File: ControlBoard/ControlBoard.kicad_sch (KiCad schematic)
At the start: 30 parts

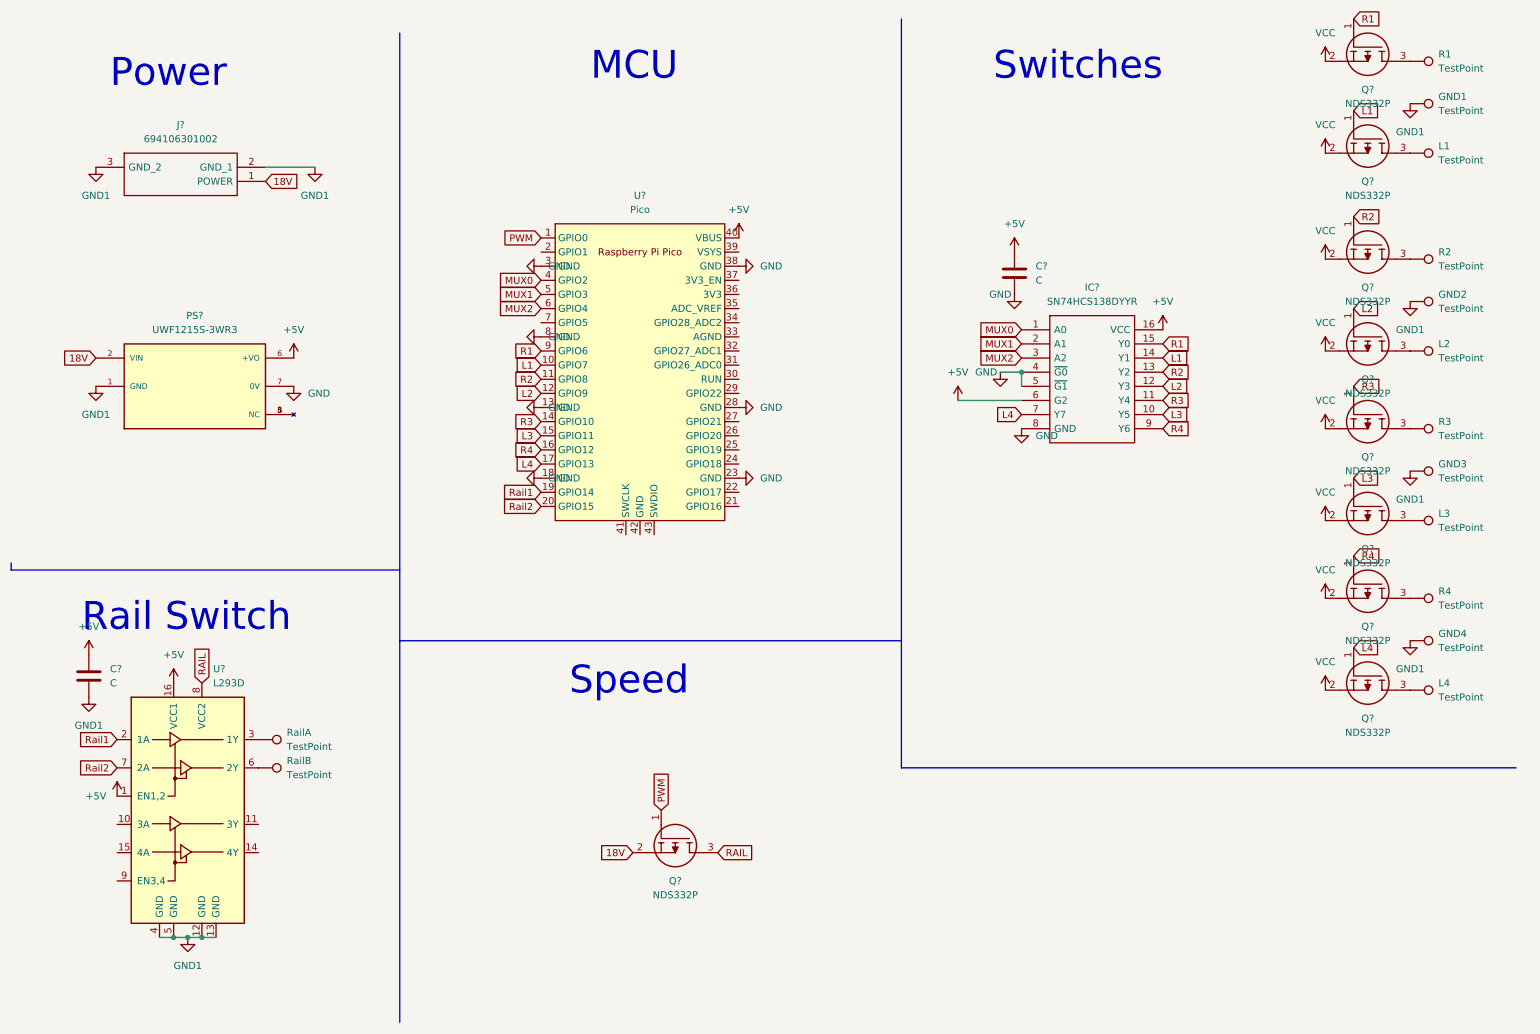
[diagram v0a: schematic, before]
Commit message: Finalized layout
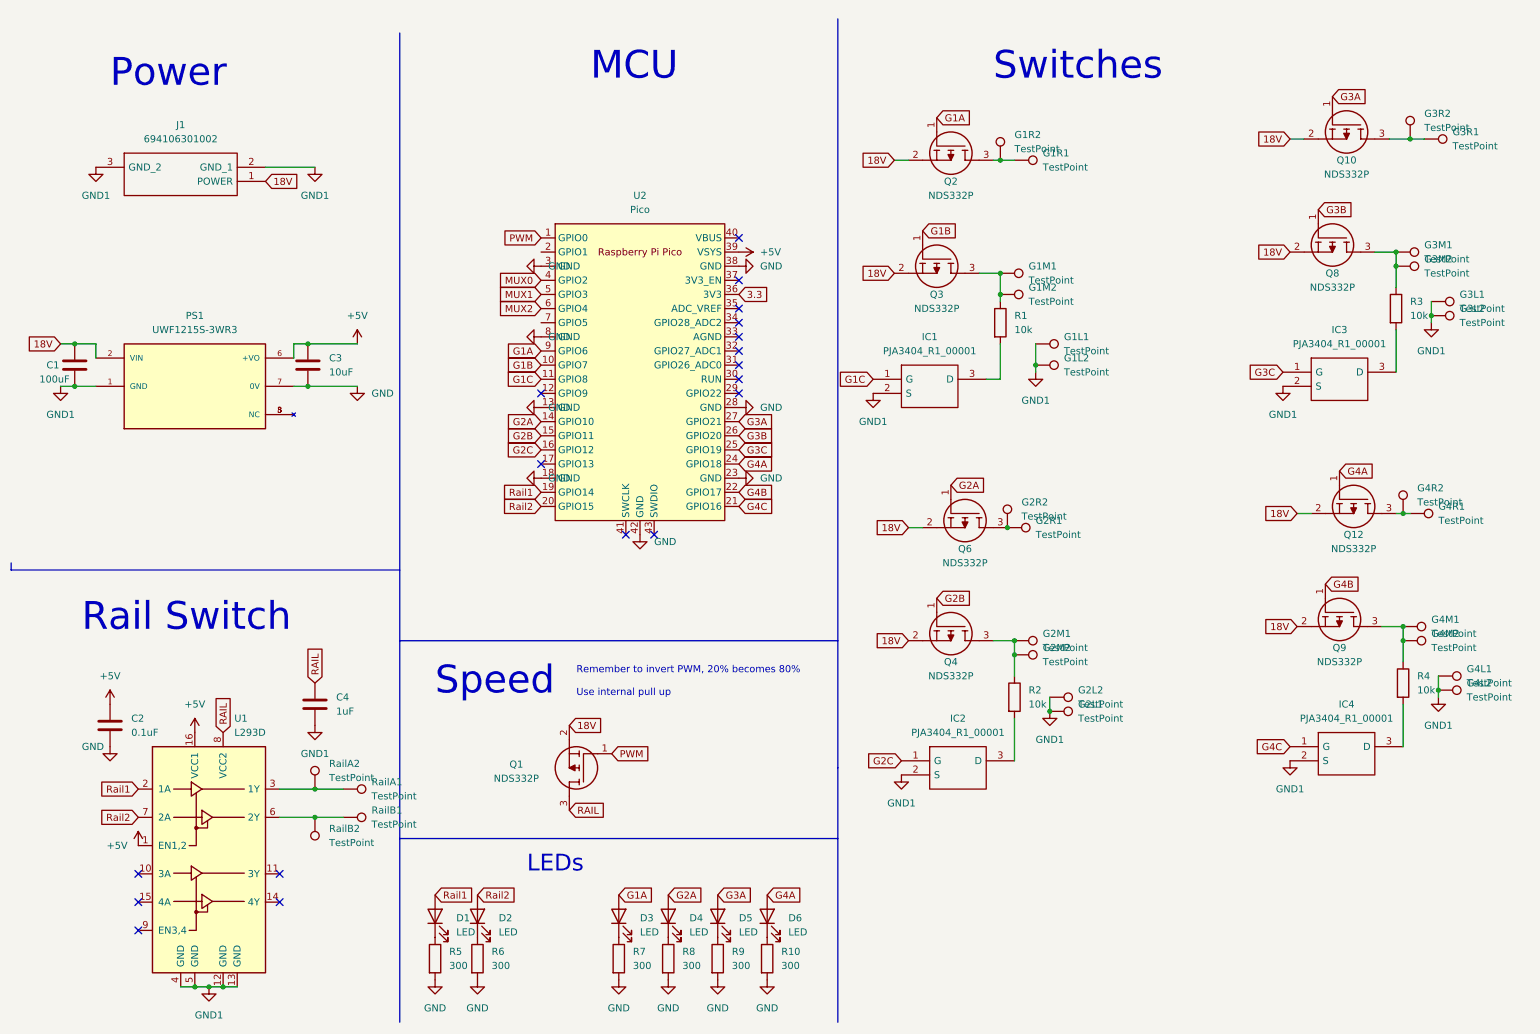
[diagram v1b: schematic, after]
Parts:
- removed C?: C, symbol Device:C
- removed GND2, GND3, GND4, L2, L3, L4, R2, R3, R4: TestPoint, symbol Connector:TestPoint
- removed IC?: SN74HCS138DYYR, SOP50P326X110-16N, symbol SamacSys_Parts:SN74HCS138DYYR
- removed Q? (x7): NDS332P, SOT95P237X112-3N, symbol SamacSys_Parts:NDS332P
- added C1: 100uF, Capacitor_THT:CP_Radial_D10.0mm_P7.50mm, symbol Device:C
- added C3: 10uF, Capacitor_THT:CP_Radial_D10.0mm_P7.50mm, symbol Device:C
- added C4: 1uF, Capacitor_THT:CP_Radial_D10.0mm_P7.50mm, symbol Device:C
- added D1, D2, D3, D4, D5, D6: LED, LED_THT:LED_D3.0mm, symbol Device:LED
- added G1L2, G1M2, G1R2, G2L1, G2L2, G2M1, G2M2, G2R1, G2R2, G3L1, G3L2, G3M1, G3M2, G3R1, G3R2, G4L1, G4L2, G4M1, G4M2, G4R1, G4R2, RailA2, RailB2: TestPoint, TestPoint:TestPoint_Pad_2.5x2.5mm, symbol Connector:TestPoint
- added IC1, IC2, IC3, IC4: PJA3404_R1_00001, SamacSys_Parts:SOT95P240X110-3N, symbol SamacSys_Parts:PJA3404_R1_00001
- added Q10, Q12, Q3, Q4, Q6, Q8, Q9: NDS332P, SamacSys_Parts:SOT95P237X112-3N, symbol SamacSys_Parts:NDS332P
- added R1, R2, R3, R4: 10k, Resistor_THT:R_Axial_DIN0204_L3.6mm_D1.6mm_P7.62mm_Horizontal, symbol Device:R
- added R10, R5, R6, R7, R8, R9: 300, Resistor_THT:R_Axial_DIN0204_L3.6mm_D1.6mm_P7.62mm_Horizontal, symbol Device:R
- C2: renamed from C?; value C -> 0.1uF; footprint (none) -> Capacitor_THT:CP_Radial_D10.0mm_P7.50mm
- G1L1: renamed from L1; footprint (none) -> TestPoint:TestPoint_Pad_2.5x2.5mm
- G1M1: renamed from GND1; footprint (none) -> TestPoint:TestPoint_Pad_2.5x2.5mm
- G1R1: renamed from R1; footprint (none) -> TestPoint:TestPoint_Pad_2.5x2.5mm
- J1: renamed from J?; footprint 694106301002_1 -> SamacSys_Parts:694106301002_1
- PS1: renamed from PS?; footprint CONV_UWF1215S-3WR3 -> UWF1215S-3WR3:CONV_UWF1215S-3WR3
- Q1, Q2: renamed from Q?; footprint SOT95P237X112-3N -> SamacSys_Parts:SOT95P237X112-3N
- RailA1: renamed from RailA; footprint (none) -> TestPoint:TestPoint_Pad_2.5x2.5mm
- RailB1: renamed from RailB; footprint (none) -> TestPoint:TestPoint_Pad_2.5x2.5mm
- U2: renamed from U?; footprint RPi_Pico:RPi_Pico_SMD_TH -> MCU_RaspberryPi_and_Boards:RPi_Pico_SMD_TH
- gave numbers to parts that had none: 1
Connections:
- net VCC is gone; now on net 18V: Q2.2
- net +5V: now also U2.39 (VSYS), C3.1; no longer U2.40 (VBUS)
- net 18V: now also C1.1, Q10.2, Q12.2, Q3.2, Q4.2, Q6.2, Q8.2, Q9.2
- net GND: now also C2.2, U2.42 (GND), C3.2, R10.2, R5.2, R6.2, R7.2, R8.2, R9.2
- net GND1: now also G1L1.1, C1.2, C4.2, G1L2.1, G2L1.1, G2L2.1, G3L1.1, G3L2.1, G4L1.1, G4L2.1, IC1.2 (S), IC2.2 (S), IC3.2 (S), IC4.2 (S); no longer C2.2, G1M1.1
- net RAIL: now also C4.1
- net Rail1: now also D1.2 (A)
- net Rail2: now also D2.2 (A)
- net at G1R1.1, Q2.3: now also G1R2.1
- net G4C: now reaches U2.21 (GPIO16)
- net G4C: now also IC4.1 (G)
- net G4B: now reaches U2.22 (GPIO17)
- net G4B: now also Q9.1
- net G4A: now reaches U2.24 (GPIO18)
- net G4A: now also D6.2 (A), Q12.1
- net G3C: now reaches U2.25 (GPIO19)
- net G3C: now also IC3.1 (G)
- net G3B: now reaches U2.26 (GPIO20)
- net G3B: now also Q8.1
- net G3A: now reaches U2.27 (GPIO21)
- net G3A: now also D5.2 (A), Q10.1
- net 3.3: now reaches U2.36 (3V3)
- net at RailB1.1, U1.6 (2Y): now also RailB2.1
- net at RailA1.1, U1.3 (1Y): now also RailA2.1
- net L1 renamed G1B
- net G1B: now also Q3.1
- net L2: no longer names the net of U2.12 (GPIO9)
- net L3 renamed G2B
- net G2B: now also Q4.1
- net L4: no longer names the net of U2.17 (GPIO13)
- net R1 renamed G1A
- net G1A: now also D3.2 (A)
- net R2 renamed G1C
- net G1C: now also IC1.1 (G)
- net R3 renamed G2A
- net G2A: now also D4.2 (A), Q6.1
- net R4 renamed G2C
- net G2C: now also IC2.1 (G)
- new net: G2R1.1, G2R2.1, Q6.3
- new net: G3R1.1, G3R2.1, Q10.3
- new net: D4.1 (K), R8.1
- new net: IC3.3 (D), R3.2
- new net: G4R1.1, G4R2.1, Q12.3
- new net: G3M1.1, G3M2.1, Q8.3, R3.1
- new net: D1.1 (K), R5.1
- new net: G1M1.1, G1M2.1, Q3.3, R1.1
- new net: IC1.3 (D), R1.2
- new net: IC2.3 (D), R2.2
- new net: G2M1.1, G2M2.1, Q4.3, R2.1
- new net: IC4.3 (D), R4.2
- new net: D5.1 (K), R9.1
- new net: D3.1 (K), R7.1
- new net: D2.1 (K), R6.1
- new net: G4M1.1, G4M2.1, Q9.3, R4.1
- new net: D6.1 (K), R10.1
- no-connect marks 0 -> 18
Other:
- note added: "LEDs"
- note added: "Remember to invert PWM, 20% becomes 80% Use internal pull up"
- moved on the sheet: C2, G1L1, G1M1, G1R1, Q1, Q2, RailA1, RailB1, U1

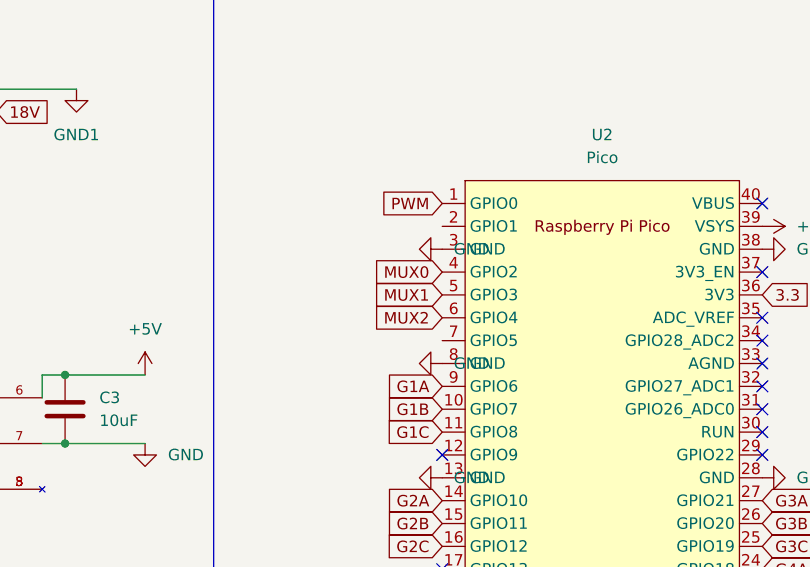
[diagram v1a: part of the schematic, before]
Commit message: Ordered
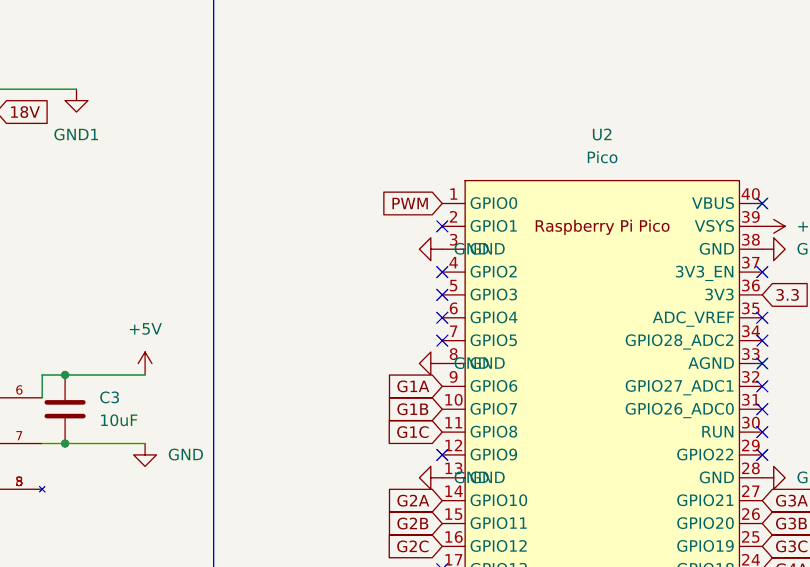
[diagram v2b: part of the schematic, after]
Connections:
- net MUX0: no longer names the net of U2.4 (GPIO2)
- net MUX1: no longer names the net of U2.5 (GPIO3)
- net MUX2: no longer names the net of U2.6 (GPIO4)
- no-connect marks 18 -> 23
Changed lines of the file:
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@@
   (no_connect (at 143.51 68.58))
   (no_connect (at 143.51 63.5))
+  (no_connect (at 107.95 71.12))
+  (no_connect (at 107.95 63.5))
+  (no_connect (at 107.95 58.42))
+  (no_connect (at 107.95 68.58))
+  (no_connect (at 107.95 66.04))
   (no_connect (at 107.95 83.82))
   (no_connect (at 107.95 96.52))
@@
     )
   )
-  (global_label "MUX0" (shape input) (at 107.95 63.5 180) (fields_autoplaced)
-    (effects (font (size 1.27 1.27)) (justify right))
-    (property "Intersheet References" "${INTERSHEET_REFS}" (id 0) (at 100.3359 63.4206 0)
-      (effects (font (size 1.27 1.27)) (justify right) hide)
-    )
-  )
-  (global_label "MUX1" (shape input) (at 107.95 66.04 180) (fields_autoplaced)
-    (effects (font (size 1.27 1.27)) (justify right))
-    (property "Intersheet References" "${INTERSHEET_REFS}" (id 0) (at 100.3359 65.9606 0)
-      (effects (font (size 1.27 1.27)) (justify right) hide)
-    )
-  )
   (global_label "RAIL" (shape input) (at 50.8 144.78 90) (fields_autoplaced)
     (effects (font (size 1.27 1.27)) (justify left))
@@
       (effects (font (size 1.27 1.27)) (justify right) hide)
     )
-  )
-  (global_label "MUX2" (shape input) (at 107.95 68.58 180) (fields_autoplaced)
-    (effects (font (size 1.27 1.27)) (justify right))
-    (property "Intersheet References" "${INTERSHEET_REFS}" (id 0) (at 100.3359 68.5006 0)
-      (effects (font (size 1.27 1.27)) (justify right) hide)
-    )
